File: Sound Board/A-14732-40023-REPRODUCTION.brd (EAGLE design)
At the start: 160 x 100 mm, 220 parts, among them P6 POWER, P7 SPEAKER, Q1 MPS3646, U1 OKI6295, U10 26LS32A, U11 26LS31, U12 27C040-150, U13 27C040-150, U14 YAMAHA 2151, U15 TIL7524, U16 74LS374, U17 74LS174, U18 16L8, U19 74LS11, U2 2064, U20 74LS139, U21 74LS14, U22 74LS74, U23 74LS74, U24 26LS31, U25 26LS32A, U26 74LS04, U28 YAMAHA 3012, U29 LM324D, U3 27C040, U30 MC3340, U31 MB3731, U32 TL084D, U33 TL084D, U4 6809E, U5 74LS374DW, U6 26LS32A, U7 26LS31, U8 74LS138, U9 74LS74, Y1 3.5749MHz, Y2 8MHz

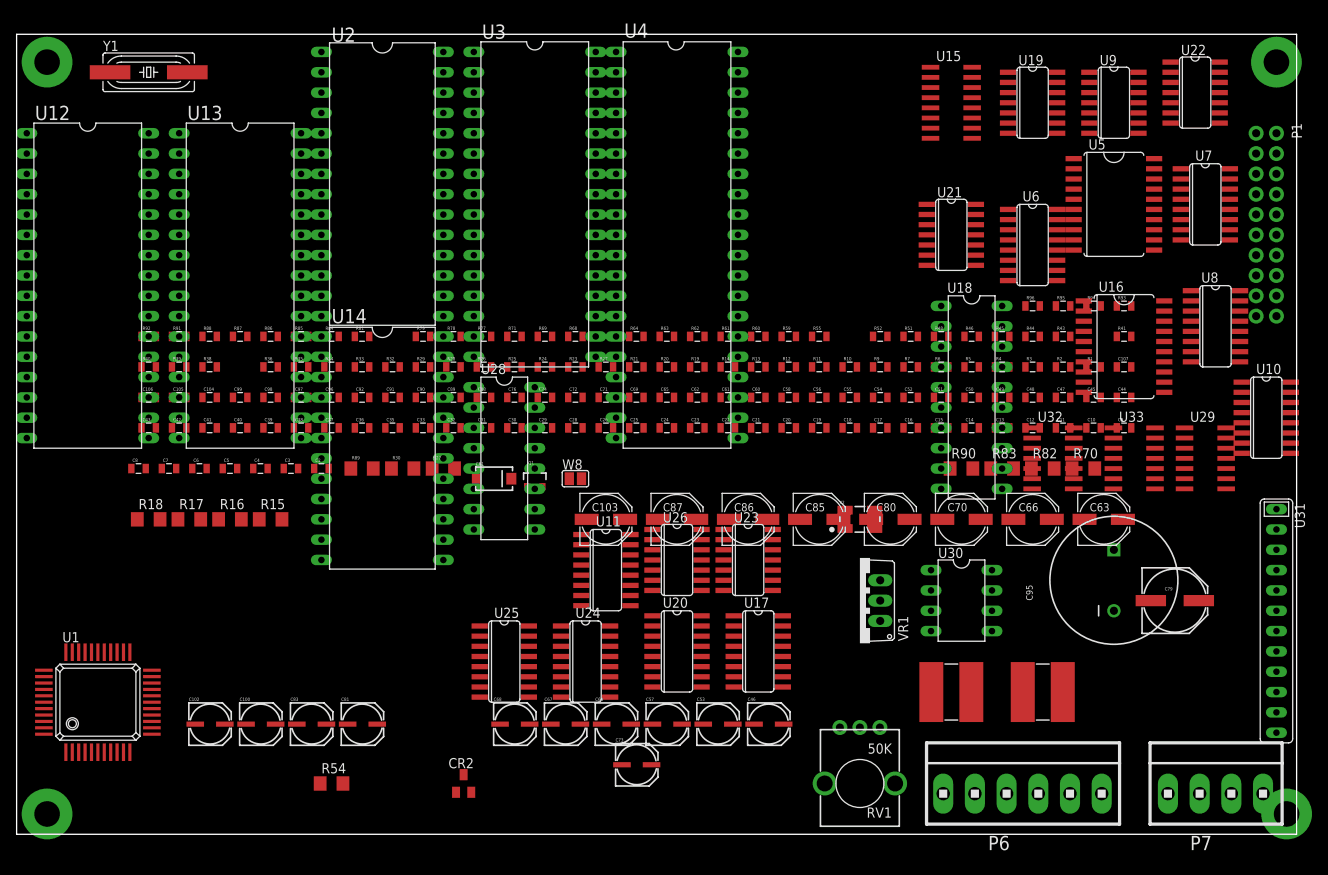
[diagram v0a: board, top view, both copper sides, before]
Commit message: layout WIP
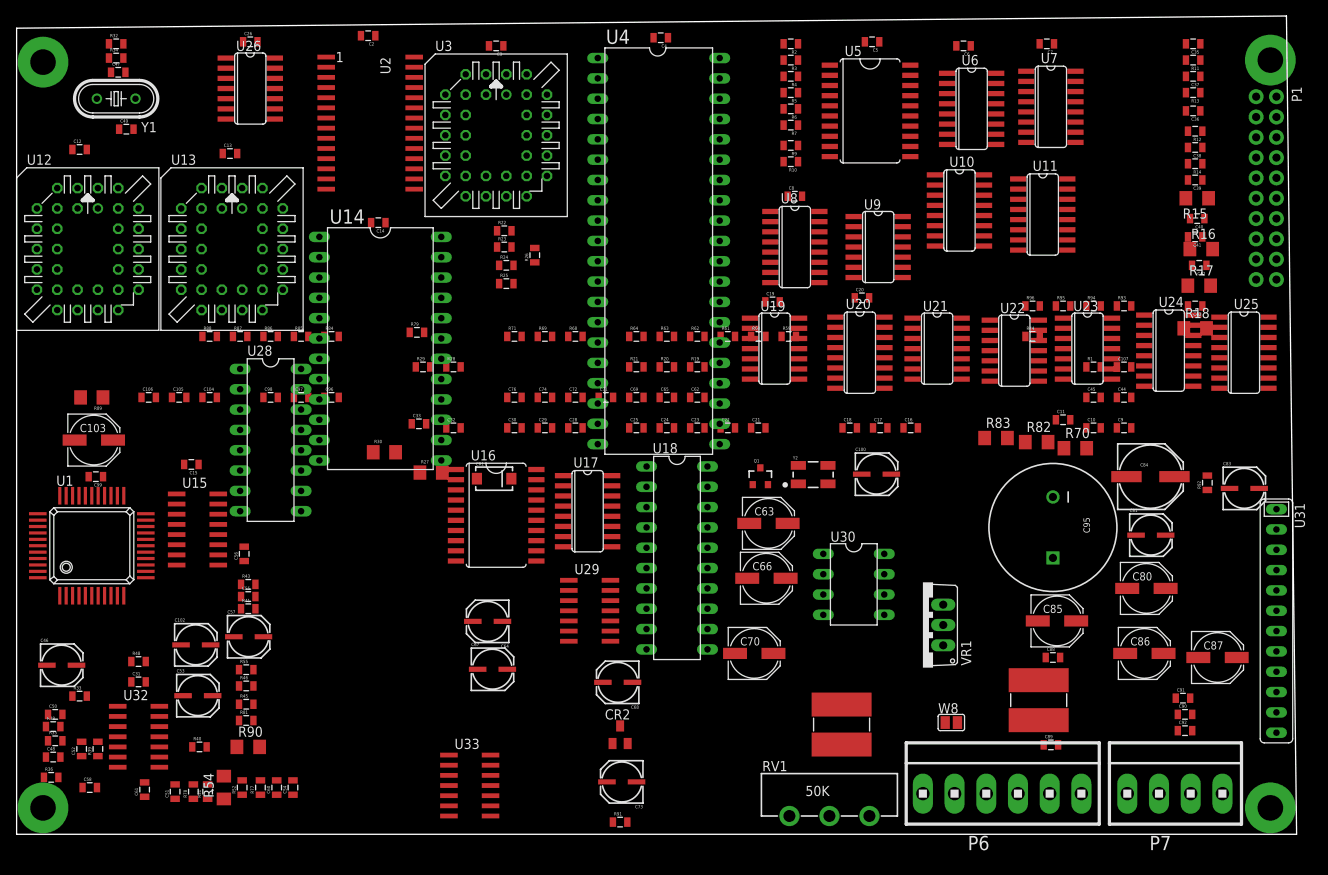
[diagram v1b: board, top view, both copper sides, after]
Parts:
- removed C79: 220uF, A-14732-40023:PANASONIC_E
- added C84: 220uF, A-14732-40023:PANASONIC_E
- RV1: device SparkFun-Electromechanical:ALPS_POT_KIT -> SparkFun-Electromechanical:POT_ALPHA_RV16AF-20
- U1: device MK-ICs:OKI6295 -> A-14732-40023:QFP44
- U12, U13, U3: device MK-ICs:27C040 -> A-14732-40023:PLCC-S32
- U14: device MK-ICs:YM2151 -> A-14732-40023:DIP24
- U18: device MK-ICs:16L8 -> A-14732-40023:DIP20N
- U2: device MK-ICs:MS6264L -> A-14732-40023:SOP28
- U28: device MK-ICs:YM3012 -> A-14732-40023:DIP16N
- Y1: device crystal:SM49 -> crystal:HC49U-V
- moved R92 133.6 mm to (148.8, 43.9), turned to 90 degrees
- moved R18 133.0 mm to (147.3, 63.2)
- moved C43 131.7 mm to (147.3, 66.0), turned to 180 degrees
- moved C48 130.4 mm to (4.57, 9.65)
- moved R17 129.6 mm to (147.8, 68.6)
- moved C42 129.1 mm to (147.8, 71.1), turned to 180 degrees
- moved R16 126.0 mm to (148.1, 73.2)
- moved C41 125.5 mm to (147.3, 74.7), turned to 180 degrees
- moved C47 124.9 mm to (12.7, 95.2)
- moved C12 124.1 mm to (7.87, 85.6)
- moved R15 122.6 mm to (147.6, 79.5), turned to 180 degrees
- moved C40 122.5 mm to (147.6, 77.0), turned to 180 degrees
- moved C7 121.9 mm to (128.8, 98.8), turned to 180 degrees
- moved C50 121.2 mm to (4.83, 15.0)
- moved C83 120.3 mm to (153.4, 43.4)
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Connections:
- net AGND: now also C84.-, RV1.1, RV1.2; no longer C79.-, RV1.P$2, RV1.P$3
- net N$87: now also RV1.3; no longer RV1.P$1
- net N$92: now also C84.+; no longer C79.+
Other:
- board size 160 x 100 mm -> 160 x 102.3 mm
